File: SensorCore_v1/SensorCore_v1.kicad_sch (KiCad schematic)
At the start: 21 parts, among them J2 M12x5 A-Type, J3 2x3 Header, J4 M12x5 A-Type, Q1 DMN2310U, U1 STM32C092KCT6, Y1 8MHz 16pF Load, Y2 8MHz 16pF Load

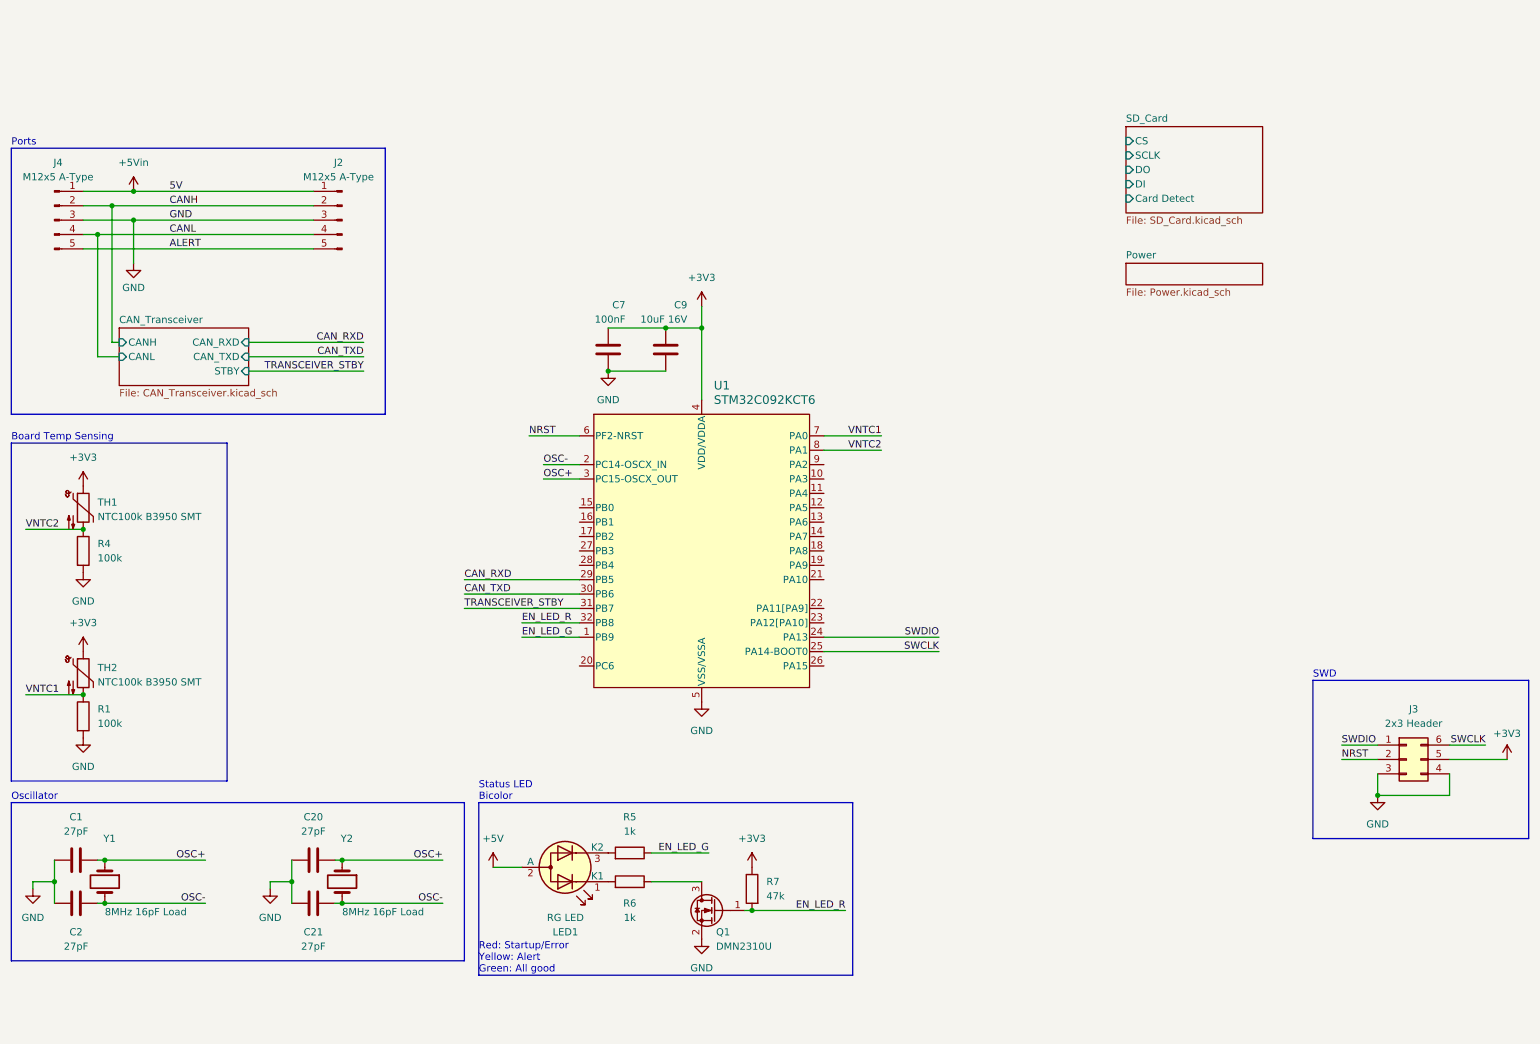
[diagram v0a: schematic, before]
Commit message: Preliminary design done
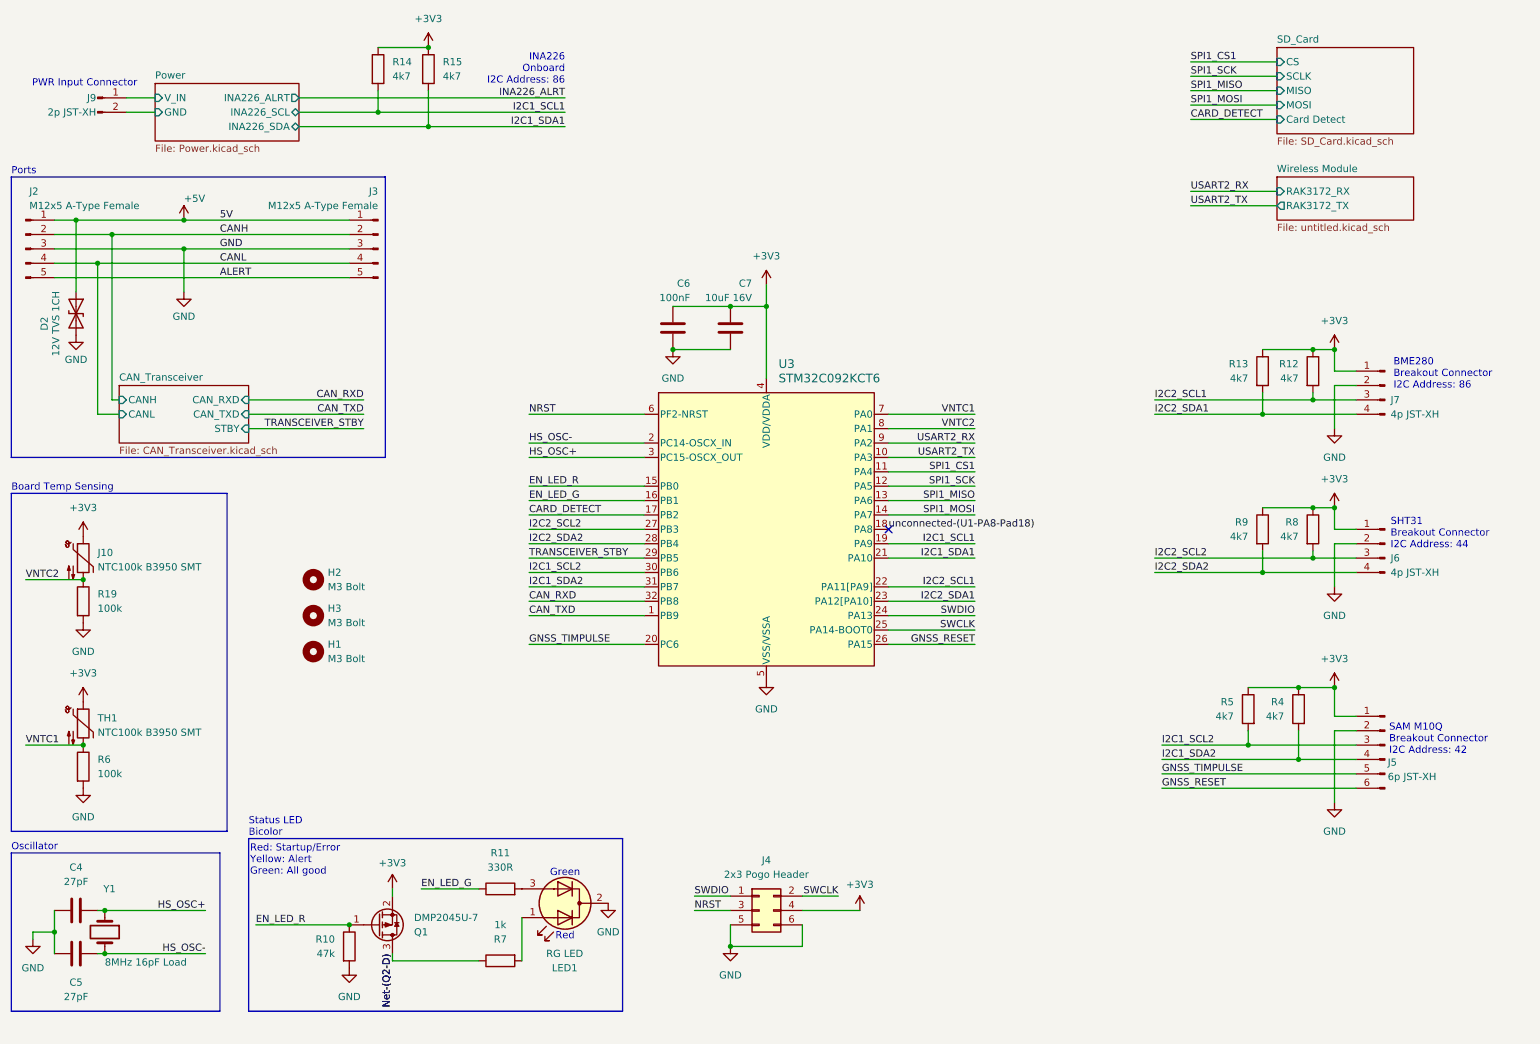
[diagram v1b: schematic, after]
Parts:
- removed C20, C21: 27pF, Capacitor_SMD:C_0603_1608Metric_Pad1.08x0.95mm_HandSolder, symbol Device:C
- removed J3: 2x3 Header, Extra_Footprints:2x03_2.54mm_DIP_pogo, symbol Connector_Generic:Conn_02x03_Counter_Clockwise
- removed LED1: RG LED, Connector_PinHeader_2.54mm:PinHeader_1x03_P2.54mm_Vertical, symbol Device:LED_Dual_KAK
- removed Q1: DMN2310U, Package_TO_SOT_SMD:SOT-23-3, symbol Transistor_FET:Q_NMOS_GSD
- removed R6: 1k, Resistor_SMD:R_0603_1608Metric_Pad0.98x0.95mm_HandSolder, symbol Device:R
- removed R7: 47k, Resistor_SMD:R_0603_1608Metric_Pad0.98x0.95mm_HandSolder, symbol Device:R
- removed Y2: 8MHz 16pF Load, Extra_Footprints:Crystal_6x3.5mm, symbol Device:Crystal
- added D2: 12V TVS 1CH, Capstone Footprints:D_SMA, symbol Project:D_TVS
- added H1, H2, H3: M3 Bolt, Capstone Footprints:MountingHole_3.2mm_M3, symbol Mechanical:MountingHole
- added J4: 2x3 Pogo Header, Capstone Footprints:PinHeader_2x03_P2.54mm_Vertical, symbol Project:Conn_02x03_Odd_Even
- added J5: 6p JST-XH, Capstone Footprints:JST_XH_B6B-XH-A_1x06_P2.50mm_Vertical, symbol Connector:Conn_01x06_Pin
- added J6, J7: 4p JST-XH, Capstone Footprints:JST_XH_B4B-XH-A_1x04_P2.50mm_Vertical, symbol Connector:Conn_01x04_Pin
- added J9: 2p JST-XH, Capstone Footprints:JST_XH_B2B-XH-A_1x02_P2.50mm_Vertical, symbol Connector:Conn_01x02_Pin
- added LED1: RG LED, Capstone Footprints:LED_D3.0mm-3, symbol Project:LED_Dual_AKA
- added Q1: DMP2045U-7, Capstone Footprints:SOT-23-3, symbol Project:Q_PMOS_GSD
- added R10: 47k, Capstone Footprints:R_0603_1608Metric_Pad0.98x0.95mm_HandSolder, symbol Project:R
- added R11: 330R, Capstone Footprints:R_0603_1608Metric_Pad0.98x0.95mm_HandSolder, symbol Project:R
- added R12, R13, R8, R9: 4k7, Capstone Footprints:R_0603_1608Metric_Pad0.98x0.95mm_HandSolder, symbol Capstone_Symbols:R
- added R14, R15: 4k7, Capstone Footprints:R_0603_1608Metric_Pad0.98x0.95mm_HandSolder, symbol Project:R
- added R4: 4k7, Capstone Footprints:R_0603_1608Metric_Pad0.98x0.95mm_HandSolder, symbol Device:R
- added R7: 1k, Capstone Footprints:R_0603_1608Metric_Pad0.98x0.95mm_HandSolder, symbol Project:R
- C4: renamed from C1; footprint Capacitor_SMD:C_0603_1608Metric_Pad1.08x0.95mm_HandSolder -> Capstone Footprints:C_0603_1608Metric_Pad1.08x0.95mm_HandSolder; symbol Device:C -> Project:C
- C5: renamed from C2; footprint Capacitor_SMD:C_0603_1608Metric_Pad1.08x0.95mm_HandSolder -> Capstone Footprints:C_0603_1608Metric_Pad1.08x0.95mm_HandSolder; symbol Device:C -> Project:C
- C6: renamed from C7; footprint Resistor_SMD:R_0603_1608Metric_Pad0.98x0.95mm_HandSolder -> Capstone Footprints:C_0603_1608Metric_Pad1.08x0.95mm_HandSolder; symbol Device:C -> Project:C; KiLib_Generator (none) -> SMD_2terminal_chip_molded
- C7: renamed from C9; footprint Capacitor_SMD:C_0805_2012Metric_Pad1.18x1.45mm_HandSolder -> Capstone Footprints:C_0805_2012Metric_Pad1.18x1.45mm_HandSolder; symbol Device:C -> Project:C
- J10: renamed from TH1; footprint Resistor_SMD:R_0603_1608Metric_Pad0.98x0.95mm_HandSolder -> Capstone Footprints:JST_XH_B2B-XH-A_1x02_P2.50mm_Vertical; symbol Device:Thermistor_NTC -> Project:Thermistor_NTC; KiLib_Generator (none) -> connector/JST
- J2: renamed from J4; value M12x5 A-Type -> M12x5 A-Type Female; footprint Extra_Footprints:M12x5_A_Circular_Connector -> Capstone Footprints:M12A05PFFRSF7003; symbol Connector:Conn_01x05_Pin -> Project:Conn_01x05_Pin
- J3: renamed from J2; value M12x5 A-Type -> M12x5 A-Type Female; footprint Extra_Footprints:M12x5_A_Circular_Connector -> Capstone Footprints:M12A05PFFRSF7003; symbol Connector:Conn_01x05_Pin -> Project:Conn_01x05_Pin
- R19: renamed from R4; footprint Resistor_SMD:R_0603_1608Metric_Pad0.98x0.95mm_HandSolder -> Capstone Footprints:R_0603_1608Metric_Pad0.98x0.95mm_HandSolder; symbol Device:R -> Project:R
- R5: value 1k -> 4k7; footprint Resistor_SMD:R_0603_1608Metric_Pad0.98x0.95mm_HandSolder -> Capstone Footprints:R_0603_1608Metric_Pad0.98x0.95mm_HandSolder; Digikey Part (none) -> RMCF0603FT4K70; KiLib_Generator (none) -> SMD_2terminal_chip_molded; Part (none) -> RMCF0603FT1K00
- R6: renamed from R1; footprint Resistor_SMD:R_0603_1608Metric_Pad0.98x0.95mm_HandSolder -> Capstone Footprints:R_0603_1608Metric_Pad0.98x0.95mm_HandSolder; symbol Device:R -> Project:R
- TH1: renamed from TH2; footprint Resistor_SMD:R_0603_1608Metric_Pad0.98x0.95mm_HandSolder -> Capstone Footprints:R_0603_1608Metric_Pad0.98x0.95mm_HandSolder; symbol Device:Thermistor_NTC -> Project:Thermistor_NTC
- U3: renamed from U1; footprint Package_QFP:LQFP-32_7x7mm_P0.8mm -> Capstone Footprints:LQFP-32_7x7mm_P0.8mm; symbol Local Symbols:STM32C092KCT6 -> Project:STM32C092KCT6
- Y1: footprint Extra_Footprints:Crystal_6x3.5mm -> Capstone Footprints:Crystal_6x3.5mm; symbol Device:Crystal -> Project:Crystal
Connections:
- net +5Vin is gone; now on net +5V: J2.1 (Pin_1), J3.1 (Pin_1)
- net +3V3: now also R5.1, J4.4 (Pin_4), J5.1 (Pin_1), J6.1 (Pin_1), J7.1 (Pin_1), Q1.2 (S), R12.1, R13.1, R14.1, R15.1, R4.1, R8.1, R9.1
- net +5V: now also D2.1 (A1)
- net CAN_RXD: now also U3.32 (PB8); no longer U3.29 (PB5)
- net CAN_TXD: now also U3.1 (PB9); no longer U3.30 (PB6)
- net EN_LED_G: now also U3.16 (PB1), R11.1; no longer R5.1, U3.1 (PB9)
- net EN_LED_R: now also U3.15 (PB0), Q1.1 (G), R10.1; no longer U3.32 (PB8)
- net GND: now also D2.2 (A2), J4.5 (Pin_5), J4.6 (Pin_6), J5.2 (Pin_2), J6.2 (Pin_2), J7.2 (Pin_2), LED1.2 (K), R10.2
- net NRST: now also J4.3 (Pin_3)
- net SWCLK: now also J4.2 (Pin_2)
- net SWDIO: now also J4.1 (Pin_1)
- net TRANSCEIVER_STBY: now also U3.29 (PB5); no longer U3.31 (PB7)
- net USART2_TX: now reaches U3.10 (PA3)
- net SPI1_CS1: now reaches U3.11 (PA4)
- net SPI1_SCK: now reaches U3.12 (PA5)
- net SPI1_MISO: now reaches U3.13 (PA6)
- net SPI1_MOSI: now reaches U3.14 (PA7)
- net CARD_DETECT: now reaches U3.17 (PB2)
- net unconnected-(U1-PA8-Pad18): now reaches U3.18 (PA8)
- net I2C1_SCL1: now reaches U3.19 (PA9)
- net I2C1_SCL1: now also R14.2
- net GNSS_TIMPULSE: now reaches U3.20 (PC6)
- net GNSS_TIMPULSE: now also J5.5 (Pin_5)
- net I2C1_SDA1: now reaches U3.21 (PA10)
- net I2C1_SDA1: now also R15.2
- net I2C2_SCL1: now reaches U3.22 (PA11[PA9])
- net I2C2_SCL1: now also J7.3 (Pin_3), R12.2
- net I2C2_SDA1: now reaches U3.23 (PA12[PA10])
- net I2C2_SDA1: now also J7.4 (Pin_4), R13.2
- net GNSS_RESET: now reaches U3.26 (PA15)
- net GNSS_RESET: now also J5.6 (Pin_6)
- net I2C2_SCL2: now reaches U3.27 (PB3)
- net I2C2_SCL2: now also J6.3 (Pin_3), R8.2
- net I2C2_SDA2: now reaches U3.28 (PB4)
- net I2C2_SDA2: now also J6.4 (Pin_4), R9.2
- net USART2_RX: now reaches U3.9 (PA2)
- net I2C1_SCL2: now reaches R5.2
- net I2C1_SCL2: now also U3.30 (PB6), J5.3 (Pin_3)
- net OSC+ renamed HS_OSC+
- net OSC- renamed HS_OSC-
- new net: LED1.1 (A1), R7.2
- new net: LED1.3 (A2), R11.2
- new net I2C1_SDA2: J5.4 (Pin_4), R4.2, U3.31 (PB7)
- new net Net-(Q2-D): Q1.3 (D), R7.1
- new net Power/GND: J9.2 (Pin_2)
- new net Power/V_IN: J9.1 (Pin_1)
- no-connect marks 0 -> 1
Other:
- added sheet Wireless Module (untitled.kicad_sch)
- sheet Power ports: added GND, INA226_ALRT, INA226_SCL, INA226_SDA, V_IN; removed none
- sheet SD_Card ports: added MISO, MOSI; removed DI, DO
- note added: "BME280 Breakout Connector I2C Address: 86"
- note added: "Green"
- note added: "INA226 Onboard I2C Address: 86"
- note added: "PWR Input Connector"
- note added: "Red"
- note added: "SAM M10Q Breakout Connector I2C Address: 42"
- note added: "SHT31 Breakout Connector I2C Address: 44"
- note removed: "SWD"
- moved on the sheet: C4, C5, C6, C7, J10, J2, J3, R19, R6, TH1, U3, Y1
